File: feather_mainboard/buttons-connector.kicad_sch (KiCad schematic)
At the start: 0 parts

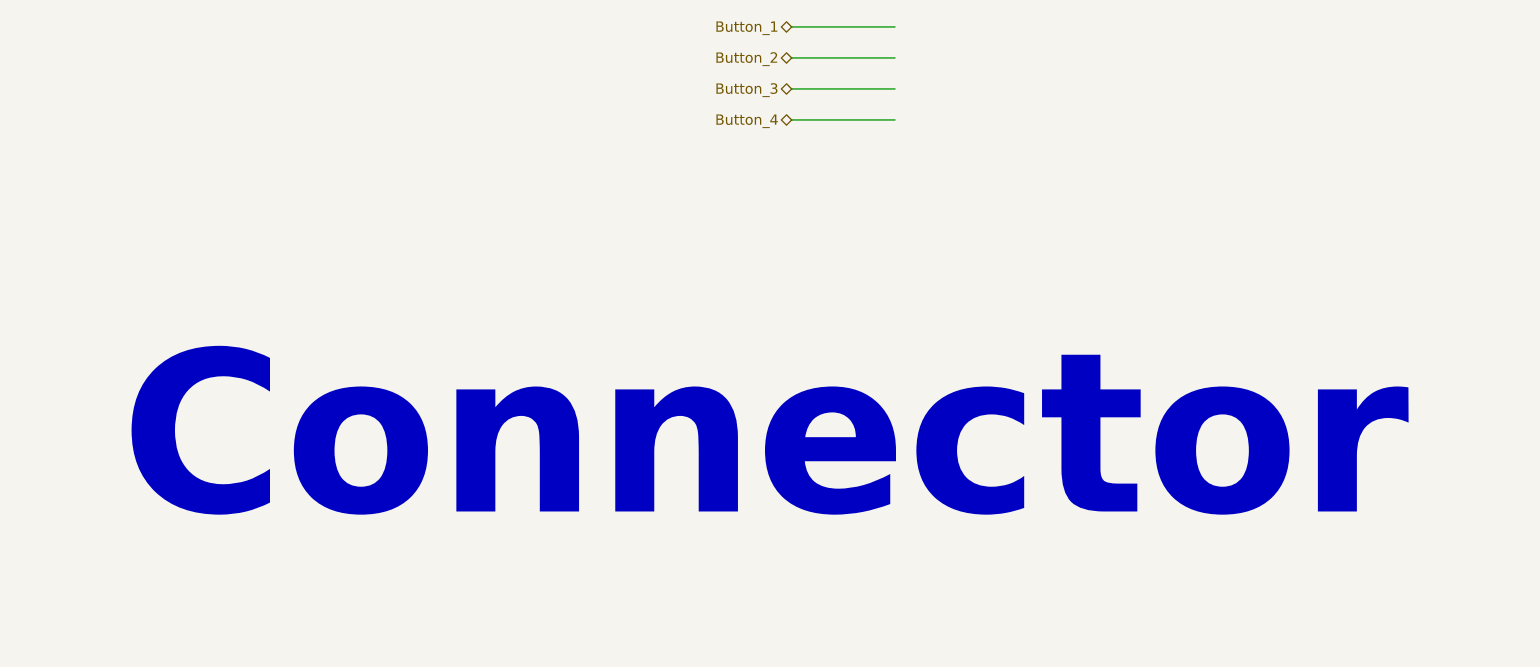
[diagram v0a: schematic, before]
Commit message: finished daughter board
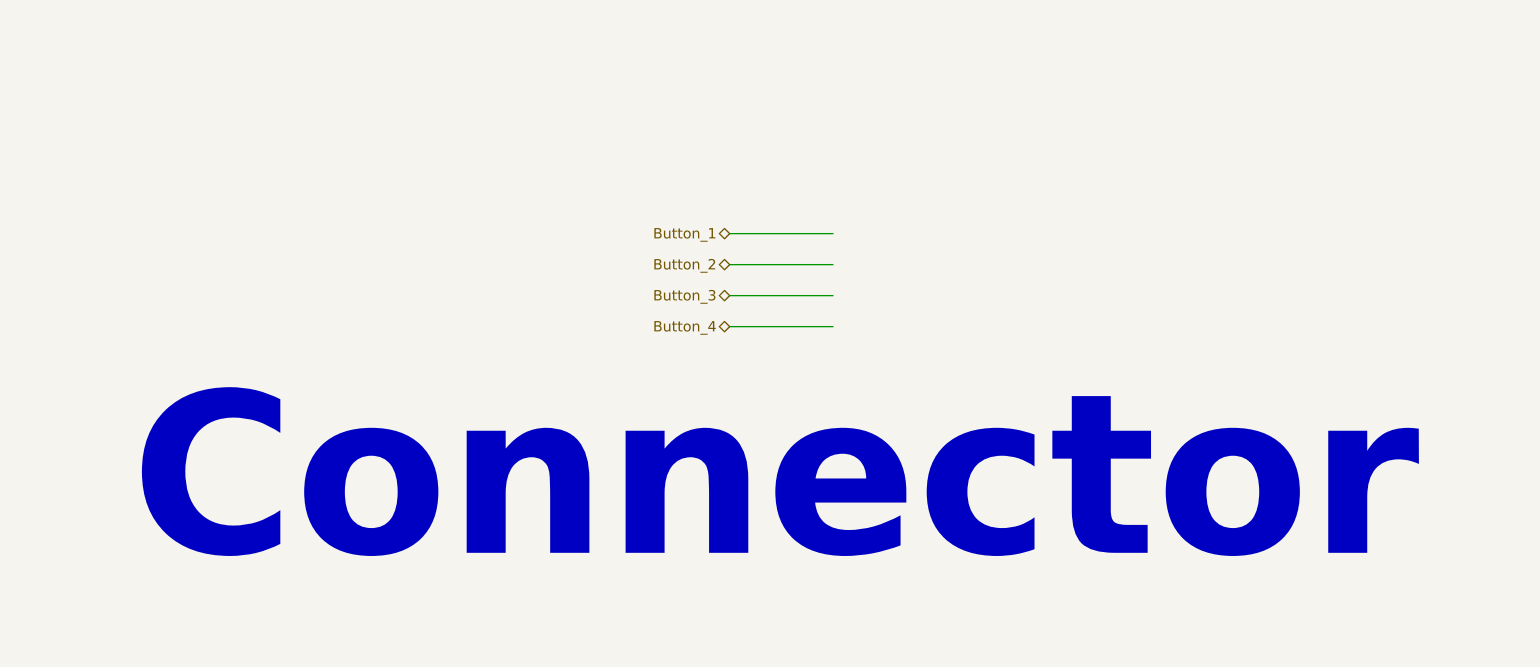
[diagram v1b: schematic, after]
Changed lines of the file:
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@@
 	(wire
 		(pts
-			(xy 152.4 62.23) (xy 165.1 62.23)
+			(xy 144.78 87.63) (xy 157.48 87.63)
 		)
 		(stroke
@@
 	(wire
 		(pts
-			(xy 152.4 50.8) (xy 165.1 50.8)
+			(xy 144.78 76.2) (xy 157.48 76.2)
 		)
 		(stroke
@@
 	(wire
 		(pts
-			(xy 152.4 54.61) (xy 165.1 54.61)
+			(xy 144.78 80.01) (xy 157.48 80.01)
 		)
 		(stroke
@@
 	(wire
 		(pts
-			(xy 152.4 58.42) (xy 165.1 58.42)
+			(xy 144.78 83.82) (xy 157.48 83.82)
 		)
 		(stroke
@@
 	(text "Connector"
 		(exclude_from_sim no)
-		(at 149.098 101.346 0)
+		(at 150.368 106.426 0)
 		(effects
 			(font
@@
 	(hierarchical_label "Button_4"
 		(shape bidirectional)
-		(at 152.4 62.23 180)
+		(at 144.78 87.63 180)
 		(fields_autoplaced yes)
 		(effects
@@
 	(hierarchical_label "Button_2"
 		(shape bidirectional)
-		(at 152.4 54.61 180)
+		(at 144.78 80.01 180)
 		(fields_autoplaced yes)
 		(effects
@@
 	(hierarchical_label "Button_3"
 		(shape bidirectional)
-		(at 152.4 58.42 180)
+		(at 144.78 83.82 180)
 		(fields_autoplaced yes)
 		(effects
@@
 	(hierarchical_label "Button_1"
 		(shape bidirectional)
-		(at 152.4 50.8 180)
+		(at 144.78 76.2 180)
 		(fields_autoplaced yes)
 		(effects

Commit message: finished mainboard design, need to do the routing
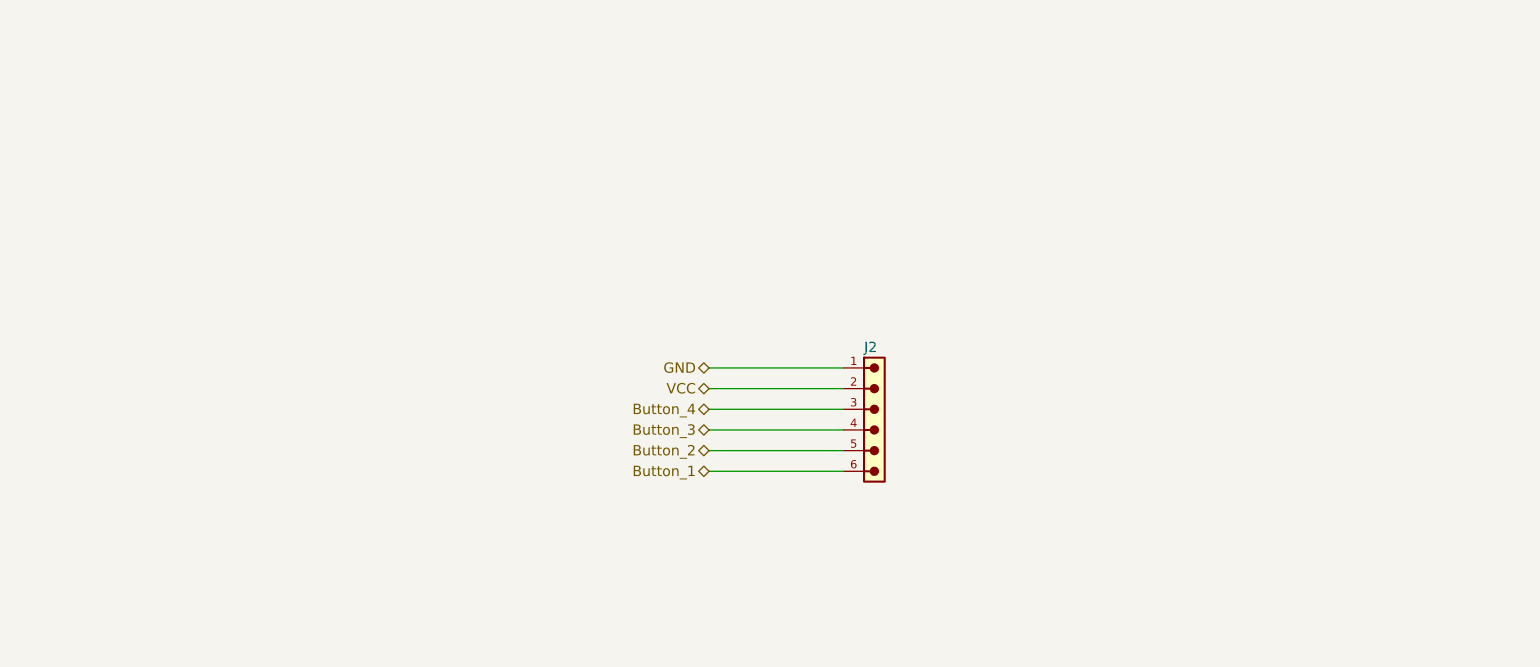
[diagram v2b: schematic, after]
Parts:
- added J2: 61900619521, Custom footprints:61900619521, symbol 61900619521:61900619521
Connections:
- net Button_1: now also J2.6
- net Button_2: now also J2.5
- net Button_3: now also J2.4
- net Button_4: now also J2.3
- new net GND: J2.1
- new net VCC: J2.2
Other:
- note removed: "Connector"

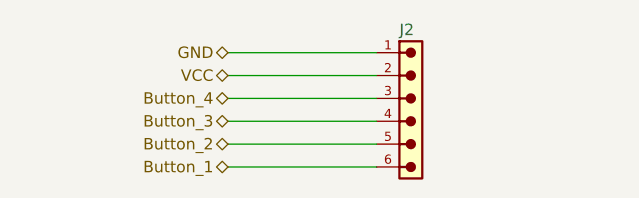
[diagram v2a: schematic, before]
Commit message: finished mainboard and daughterboard
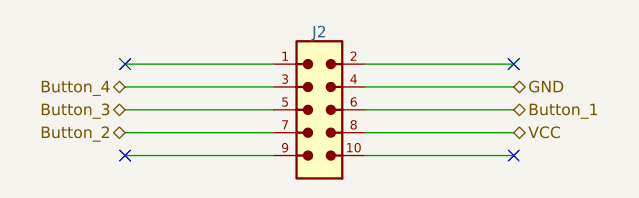
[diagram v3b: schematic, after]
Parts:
- removed J2: 61900619521, Custom footprints:61900619521, symbol 61900619521:61900619521
- added J2: 62501021721, Custom footprints:62501021721, symbol 6250XX21721_62501021721:6250XX21721_62501021721
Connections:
- net Button_1: now also J2.6
- net Button_2: now also J2.7
- net Button_3: now also J2.5
- net Button_4: now also J2.3
- net GND: now also J2.4
- net VCC: now also J2.8
- no-connect marks 0 -> 4
